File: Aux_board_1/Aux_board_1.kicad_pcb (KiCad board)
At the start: 2 copper layers, 60 parts, among them J1 P03d, J2 P11a, J3 P10a, J4 PHI_ENC, J5 PHI_LIM_CLW, J6 PHI_LIM_CCW, J7 PHI_HOME, Q1 BSS138, Q10 BSS84, Q2 BSS84, Q3 BSS138, Q4 BSS84, Q5 BSS138, Q6 BSS84, Q7 BSS138, Q8 BSS84, Q9 BSS138, U2 AMS1117-3.3

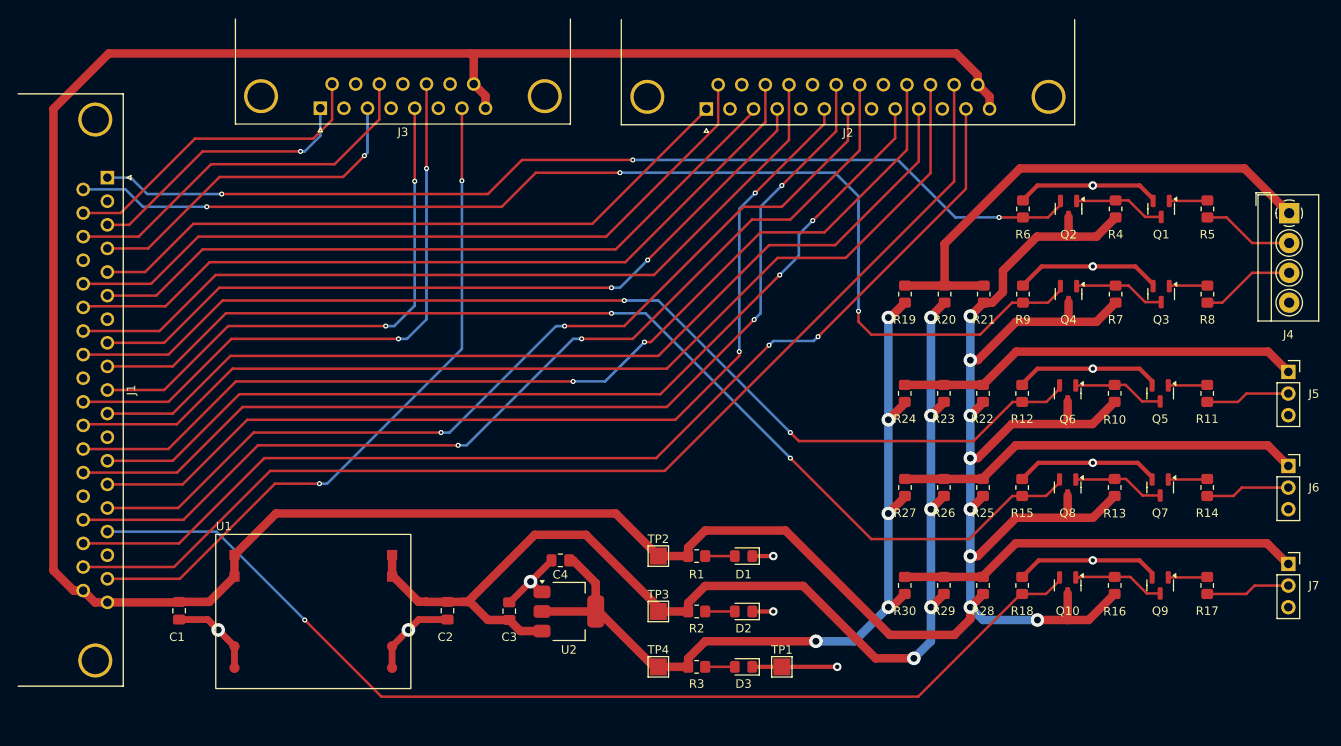
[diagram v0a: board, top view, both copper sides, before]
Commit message: finished designing Board 1
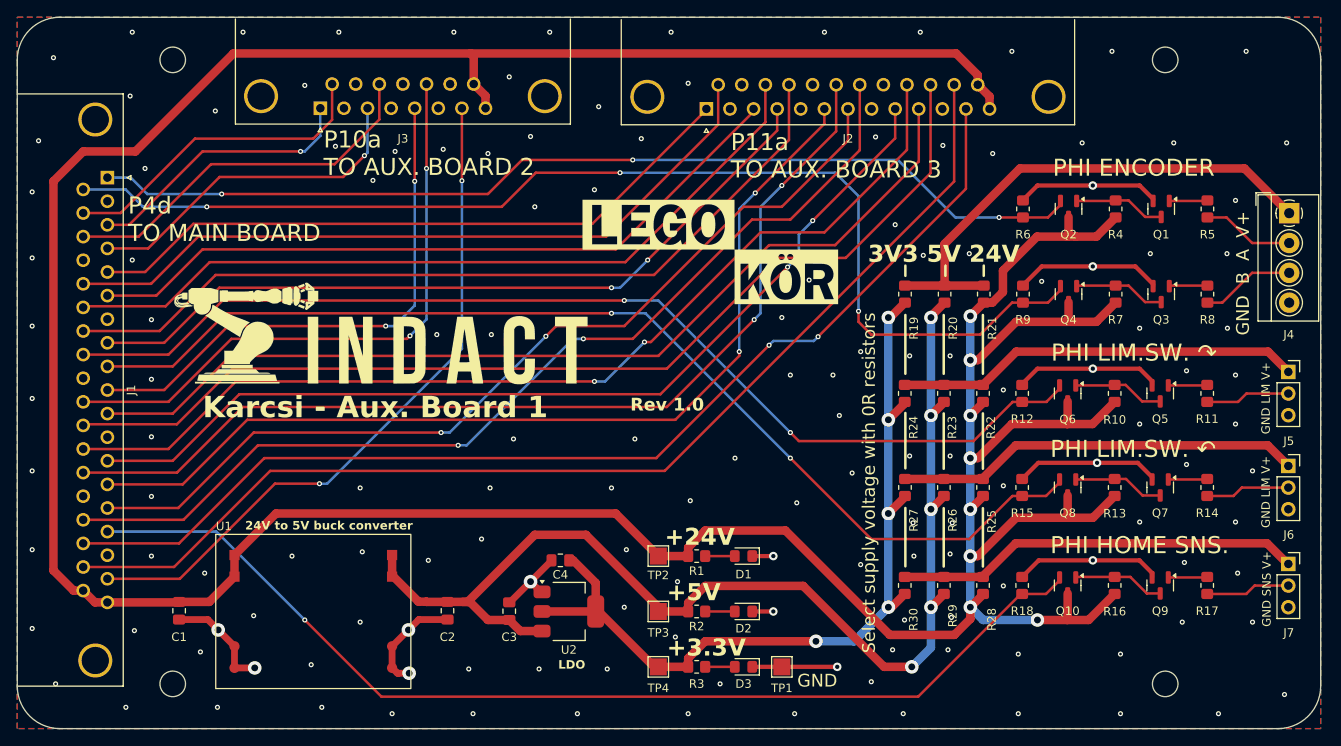
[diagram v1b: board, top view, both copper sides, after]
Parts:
- added MH1: MountingHole_3mm, MountingHole:MountingHole_3mm, F.Cu at (55.0, 53.2)
- added MH2: MountingHole_3mm, MountingHole:MountingHole_3mm, F.Cu at (171.5, 53.2)
- added MH3: MountingHole_3mm, MountingHole:MountingHole_3mm, F.Cu at (55.0, 126.5)
- added MH4: MountingHole_3mm, MountingHole:MountingHole_3mm, F.Cu at (171.5, 126.5)
- added REF**: INDACTlogo, LEGOkor:INDACTlogo, F.Cu at (79.9, 85.7)
- added REF**: LEGOkorLogo, LEGOkor:LEGOkorLogo, F.Cu at (117.6, 77.3)
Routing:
- net +24V: track 459.7 -> 454.8 mm
- net GND: track 130.1 -> 134.8 mm, vias 11 -> 150
- net +5V: track 138.3 -> 139.5 mm
- added copper zone on B.Cu, net GND
- added copper zone on F.Cu, net GND
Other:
- board outline added: 153 x 83.5 mm
- board text added: "+24V"
- board text added: "+3.3V"
- board text added: "+5V"
- board text added: "24V to 5V buck converter"
- board text added: "3V3 5V 24V"
- board text added: "GND"
- board text added: "GND B A V+"
- board text added: "GND LIM V+"
- board text added: "GND SNS V+"
- board text added: "Karcsi - Aux. Board 1"
- board text added: "LDO"
- board text added: "P10a TO AUX. BOARD 2"
- board text added: "P11a TO AUX. BOARD 3"
- board text added: "P4d TO MAIN BOARD"
- board text added: "PHI ENCODER"
- board text added: "PHI HOME SNS."
- board text added: "PHI LIM.SW. ↶"
- board text added: "PHI LIM.SW. ↷"
- board text added: "Rev 1.0"
- board text added: "Select supply voltage with 0R resistors"

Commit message: Finished Board 2 schematic
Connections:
- net /PHIL_LIM_CLW_IN renamed /PHI_LIM_CLW_IN
